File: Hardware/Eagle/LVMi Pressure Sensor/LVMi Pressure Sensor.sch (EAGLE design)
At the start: 33 parts, among them J1 POWER_JACKPJ-102AH, SW1 SWITCH-RA-800BWSP9SM6RE, U2 Sensiron SDP800, U3 SN74LV1T34DBVR, U4 ATTINY1624-SSU, U5 TXB0102DCURVSSOP8

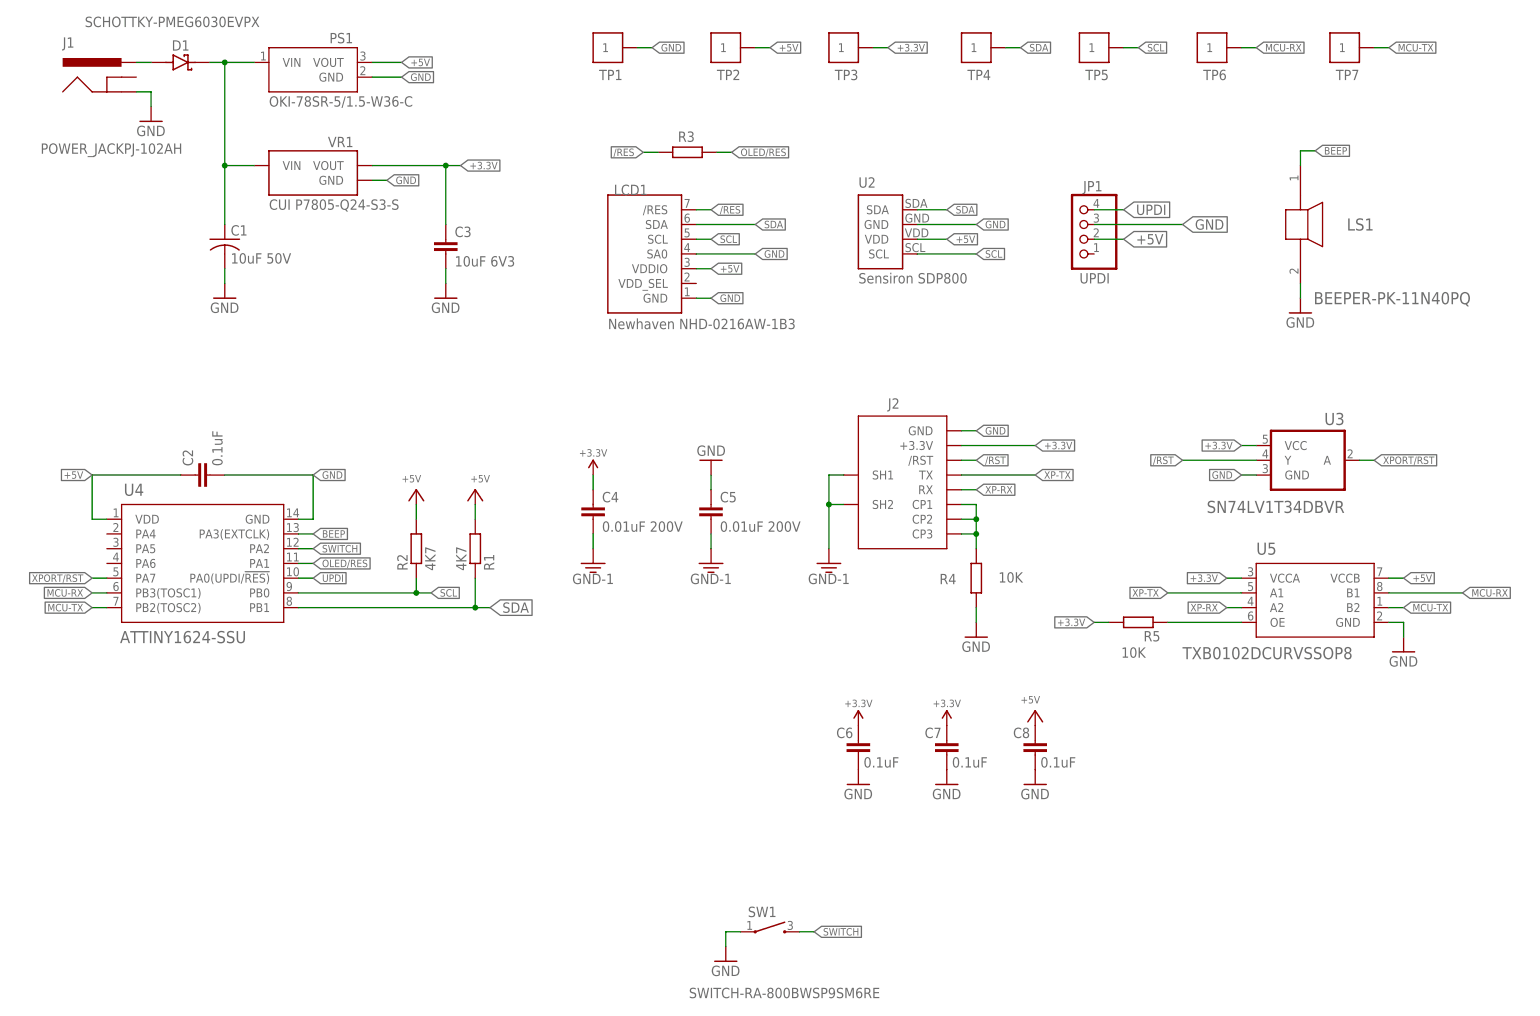
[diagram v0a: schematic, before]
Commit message: WIP
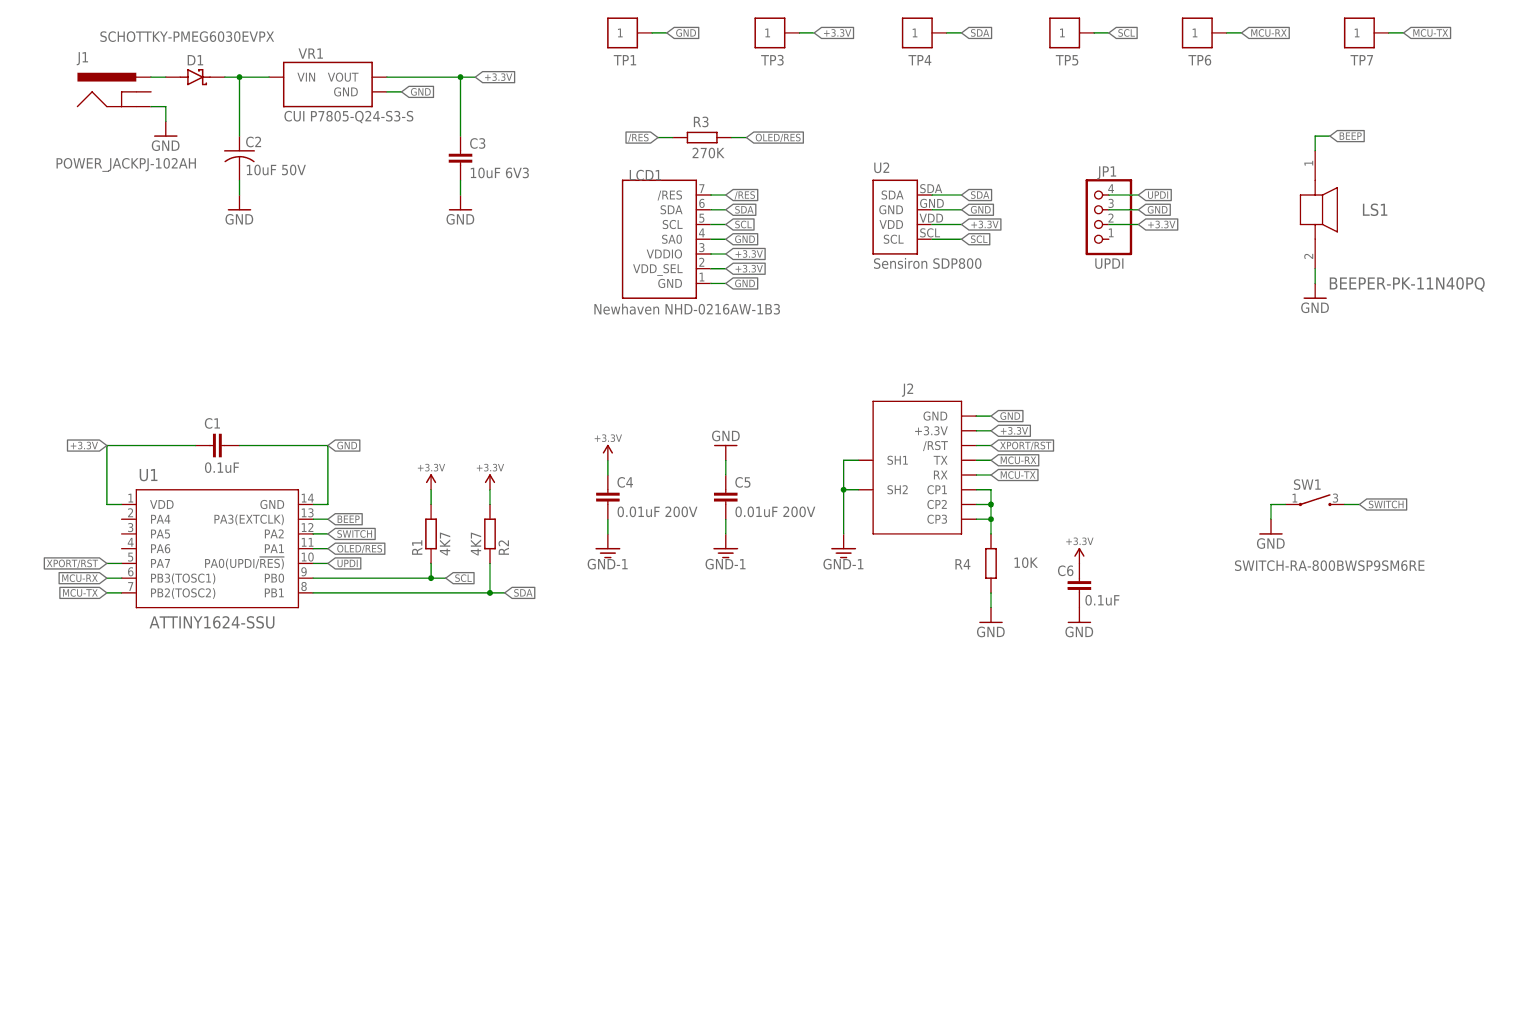
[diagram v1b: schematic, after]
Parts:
- removed C7, C8: 0.1uF, AUmlib:C-EUC0805
- removed PS1: OKI-78SR-5/1.5-W36-C, AUmlib:OKI-78SR-5/1.5-W36-C
- removed R5: 10K, AUmlib:R-EU_R0805
- removed TP2: +5V, AUmlib:TP5000-TESTPOINT-RED
- removed U3: SN74LV1T34DBVR, AUmlib:SN74LV1T34DBVR
- removed U4: ATTINY1624-SSU, AUmlib:ATTINY1624-SSUSOIC150-14_MCH-M
- removed U5: TXB0102DCURVSSOP8, AUmlib:TXB0102DCURVSSOP8
- added U1: ATTINY1624-SSU, AUmlib:ATTINY1624-SSUSOIC150-14_MCH-M
- C1: value 10uF 50V -> 0.1uF; device AUmlib:C-USC1210 -> AUmlib:C-EUC0805
- C2: value 0.1uF -> 10uF 50V; device AUmlib:C-EUC0805 -> AUmlib:C-USC1210
- R3: value (none) -> 270K
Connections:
- removed net +5V: C2.1, C8.2, JP1.2, LCD1.VDDIO, PS1.VOUT, R1.2, R2.2, TP2.1, U2.VDD, U4.VDD, U5.VCCB
- removed net /RST: J2./RST, U3.Y
- removed net OE: R5.1, U5.OE
- removed net XP-RX: J2.RX, U5.A2
- removed net XP-TX: J2.TX, U5.A1
- net +3.3V: now also C1.1, JP1.2, LCD1.VDDIO, LCD1.VDD_SEL, R1.2, R2.2, U1.VDD, U2.VDD; no longer C7.2, R5.2, U3.VCC, U5.VCCA
- net BEEP: now also U1.PA3(EXTCLK); no longer U4.PA3(EXTCLK)
- net GND: now also U1.GND; no longer C7.1, C8.1, PS1.GND, U3.GND, U4.GND, U5.GND
- net MCU-RX: now also J2.TX, U1.PB3(TOSC1); no longer U4.PB3(TOSC1), U5.B1
- net MCU-TX: now also J2.RX, U1.PB2(TOSC2); no longer U4.PB2(TOSC2), U5.B2
- net OLED/RES: now also U1.PA1; no longer U4.PA1
- net SCL: now also R1.1, U1.PB0; no longer R2.1, U4.PB0
- net SDA: now also R2.1, U1.PB1; no longer R1.1, U4.PB1
- net SWITCH: now also U1.PA2; no longer U4.PA2
- net UPDI: now also U1.PA0(UPDI/!RES); no longer U4.PA0(UPDI/!RES)
- net VIN: now also C2.1; no longer C1.1, PS1.VIN
- net XPORT/RST: now also J2./RST, U1.PA7; no longer U3.A, U4.PA7
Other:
- note added: "Display Switch"
- moved on the sheet: C1, C2, C3, C4, C5, C6, D1, J1, J2, JP1, LCD1, LS1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
